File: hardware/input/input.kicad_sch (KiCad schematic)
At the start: 0 parts

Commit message: rearranging shared files and input board beginnings
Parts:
- added C1, C4: 100nF, Capacitor_SMD:C_0402_1005Metric, symbol Device:C
- added C2, C3: 4.7µF, Capacitor_SMD:C_0603_1608Metric, symbol Device:C
- added CGQ1: IRM-H638T/TR2, easyeda2kicad:SENSOR-SMD_IRM-H638T-TR2-TL, symbol easyeda2kicad:IRM-H638T_TR2
- added H1, H2, H3, H4: MountingHole, MountingHole:MountingHole_3.2mm_M3_Pad, symbol Mechanical:MountingHole
- added R1: 100Ω, Resistor_SMD:R_0603_1608Metric, symbol Device:R_US
- added SW1, SW2, SW3, SW4, SW5: EVP-ASAC1A, easyeda2kicad:SW-SMD_PANASONIC_EVPASXXX, symbol easyeda2kicad:EVP-ASAC1A
- added SW6: CL-SB-13A-02T, easyeda2kicad:SW-SMD_CL-SB-13A-0X, symbol easyeda2kicad:CL-SB-13A-02T
- added U1: MCP23008T-E/SS, easyeda2kicad:SSOP-20_L7.2-W5.3-P0.65-LS7.8-TL, symbol easyeda2kicad:MCP23008T-E_SS
- added USBC1: TYPE-C-31-M-12, easyeda2kicad:USB-C_SMD-TYPE-C-31-M-12_1, symbol easyeda2kicad:TYPE-C-31-M-12
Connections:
- new net: C1.1, C2.2, CGQ1.4 (VCC), R1.1
- new net +3.3V: C3.2, C4.1, R1.2, U1.20 (VDD), U1.6 (~{RESET}), USBC1.A4B9 (VBUS), USBC1.B4A9 (VBUS)
- new net BTN CENTER: SW5.1, U1.16 (GP4)
- new net BTN DOWN: SW2.1, U1.13 (GP1)
- new net BTN LEFT: SW3.1, U1.14 (GP2)
- new net BTN RIGHT: SW4.1, U1.15 (GP3)
- new net BTN UP: SW1.1, U1.12 (GP0)
- new net GND: C1.2, C2.1, C3.1, C4.2, CGQ1.1 (GND), CGQ1.2 (GND), SW1.2, SW2.2, SW3.2, SW4.2, SW5.2, SW6.3, U1.3 (A2), U1.4 (A1), U1.5 (A0), U1.9 (VSS), USBC1.1 (EH), USBC1.2 (EH), USBC1.3 (EH), USBC1.4 (EH), USBC1.A1B12 (GND), USBC1.B1A12 (GND)
- new net IR SENSOR DATA: CGQ1.3 (VOUT), USBC1.A8 (SBU1), USBC1.B8 (SBU2)
- new net SOUND REACTIVE OFF: SW6.4, U1.18 (GP6)
- new net SOUND REACTIVE ON: SW6.1, U1.17 (GP5)
- new net USB-C CC1&CC2: U1.8 (INT), USBC1.A5 (CC1), USBC1.B5 (CC2)
- new net USB-C D+: U1.2 (SDA), USBC1.A6 (DP1), USBC1.B6 (DP2)
- new net USB-C D-: U1.1 (SCL), USBC1.A7 (DN1), USBC1.B7 (DN2)
- no-connect marks 0 -> 4

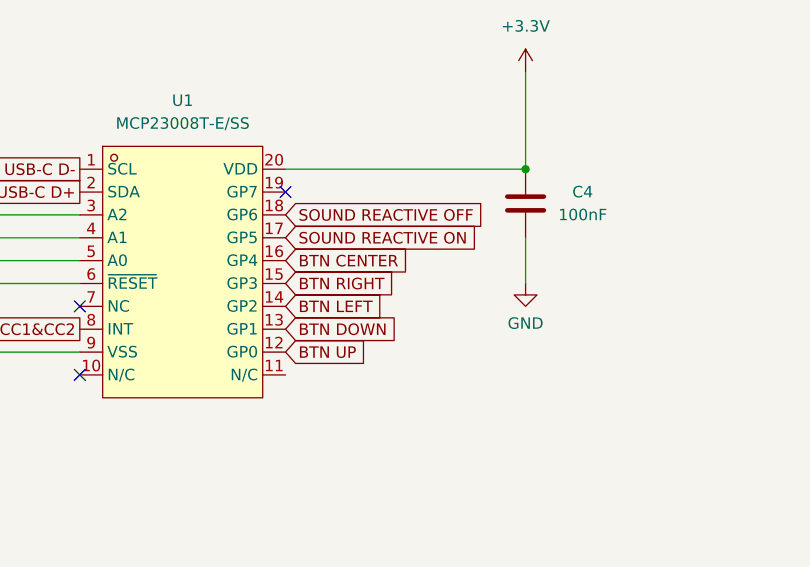
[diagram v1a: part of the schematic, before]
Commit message: a few more changes for the input board
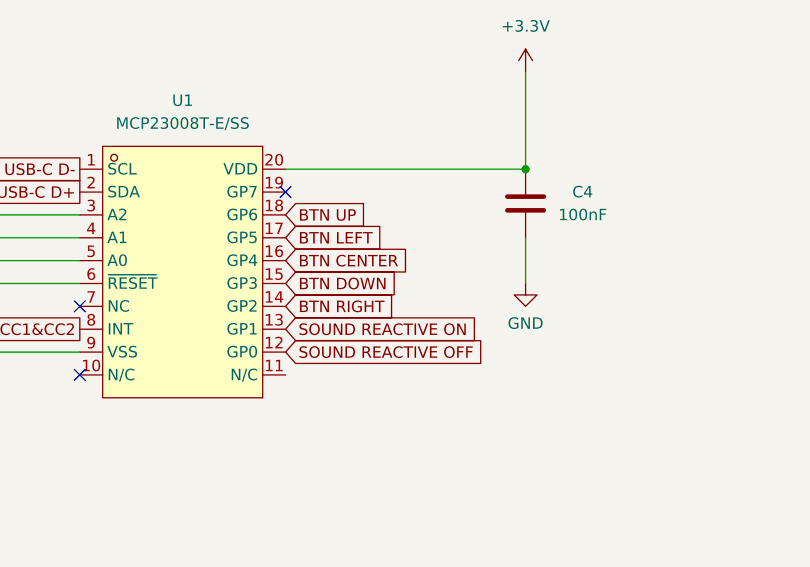
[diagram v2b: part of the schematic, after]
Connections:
- net BTN DOWN: now also U1.15 (GP3); no longer U1.13 (GP1)
- net BTN LEFT: now also U1.17 (GP5); no longer U1.14 (GP2)
- net BTN RIGHT: now also U1.14 (GP2); no longer U1.15 (GP3)
- net BTN UP: now also U1.18 (GP6); no longer U1.12 (GP0)
- net SOUND REACTIVE OFF: now also U1.12 (GP0); no longer U1.18 (GP6)
- net SOUND REACTIVE ON: now also U1.13 (GP1); no longer U1.17 (GP5)
